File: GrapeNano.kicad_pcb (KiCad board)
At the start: 2 copper layers, 18.5 x 43.7 mm, 31 parts, among them P1 USB_OTG, P2 ICSP, SW1 SW_Push, U1 LM1117-5.0, U2 CH340G, U3 ATMEGA328P-AU, Y1 12MHz, Y2 16Mhz

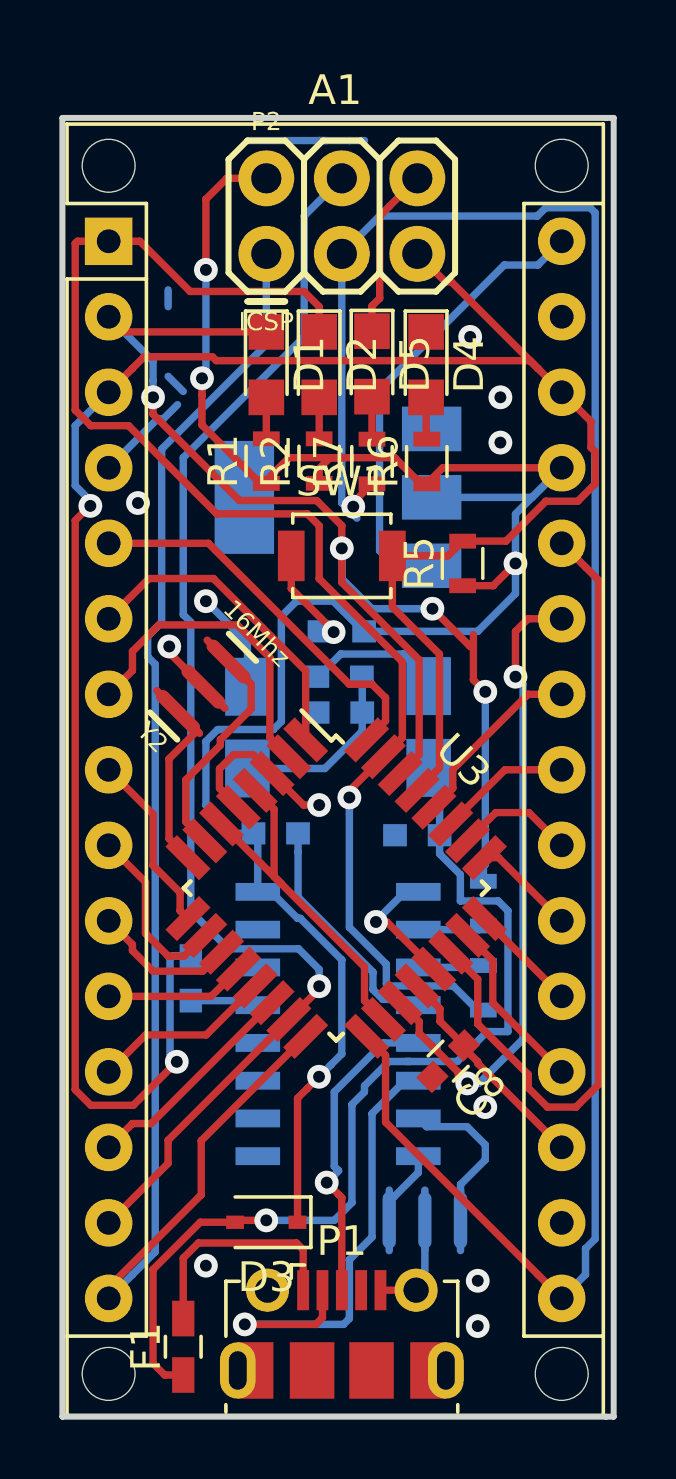
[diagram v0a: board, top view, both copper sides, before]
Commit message: 1 net
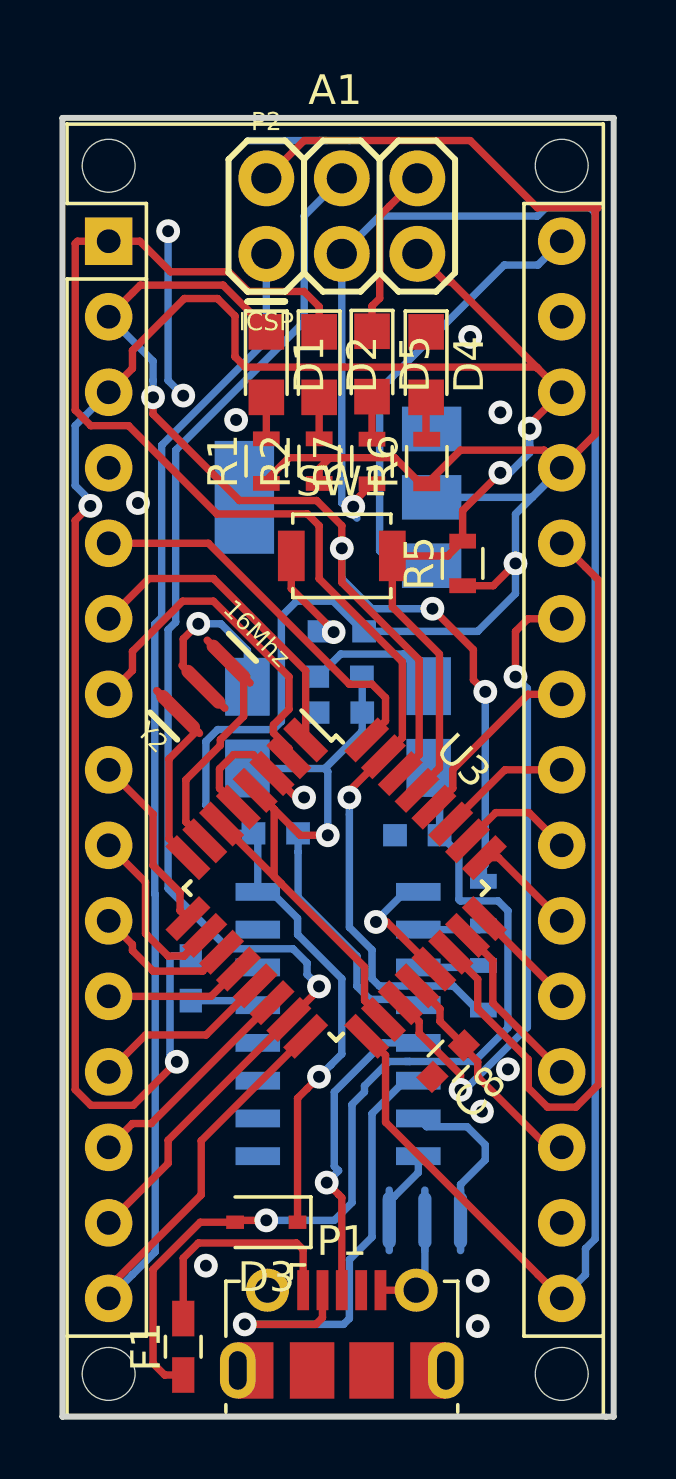
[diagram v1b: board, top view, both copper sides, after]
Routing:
- net +5V: track 71.6 -> 81.0 mm, vias 4 -> 2
- net Net-(C6-Pad1): track 18.6 -> 23.9 mm, vias 0 -> 1
- net GND: track 36.5 -> 39.0 mm, vias 12 -> 14
- net (no net): track 5.44 -> 4.16 mm
- net D4: track 10.8 -> 11.9 mm
- net RESET: track 75.1 -> 76.0 mm, vias 2 -> 4
